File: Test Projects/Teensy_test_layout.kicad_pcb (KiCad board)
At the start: 2 copper layers, 203.2 x 101.6 mm, 106 parts, among them P1 CONN_01X02, P10 CONN_01X08, P11 CONN_01X08, P12 COLUMNS, P13 CONN_01X08, P14 CONN_01X08, P15 CONN_01X08, P16 CONN_01X08, P17 CONN_01X08, P18 CONN_01X08, P19 CONN_01X08, P2 CONN_01X07, P20 CONN_01X08, P3 CONN_01X08, P4 CONN_01X08, P5 CONN_01X08, P6 CONN_01X08, P7 ROWS, P8 CONN_01X08, P9 CONN_01X08, U1 LDO-adj-4term, U10 SF-4052, U11 SF-4052, U12 SF-4052, U13 SF-4052, U14 SF-4052, U15 SF-4052, U16 SF-4052, U17 SF-4052, U18 SF-74HC595, U19 SF-74HC595, U2 Teensy_3.2, U20 SF-74HC595, U21 SF-74HC595, U22 SF-74HC595, U23 SF-74HC595, U24 SF-74HC595, U25 SF-74HC595, U26 SF-74HC595, U27 SF-74HC595, U3 LDO-adj-4term, U4 SGTL5000, U5 SF-MicroSD-12term, U6 LDO-adj-4term, U7 2N168, U8 SF-4052, U9 SF-4052

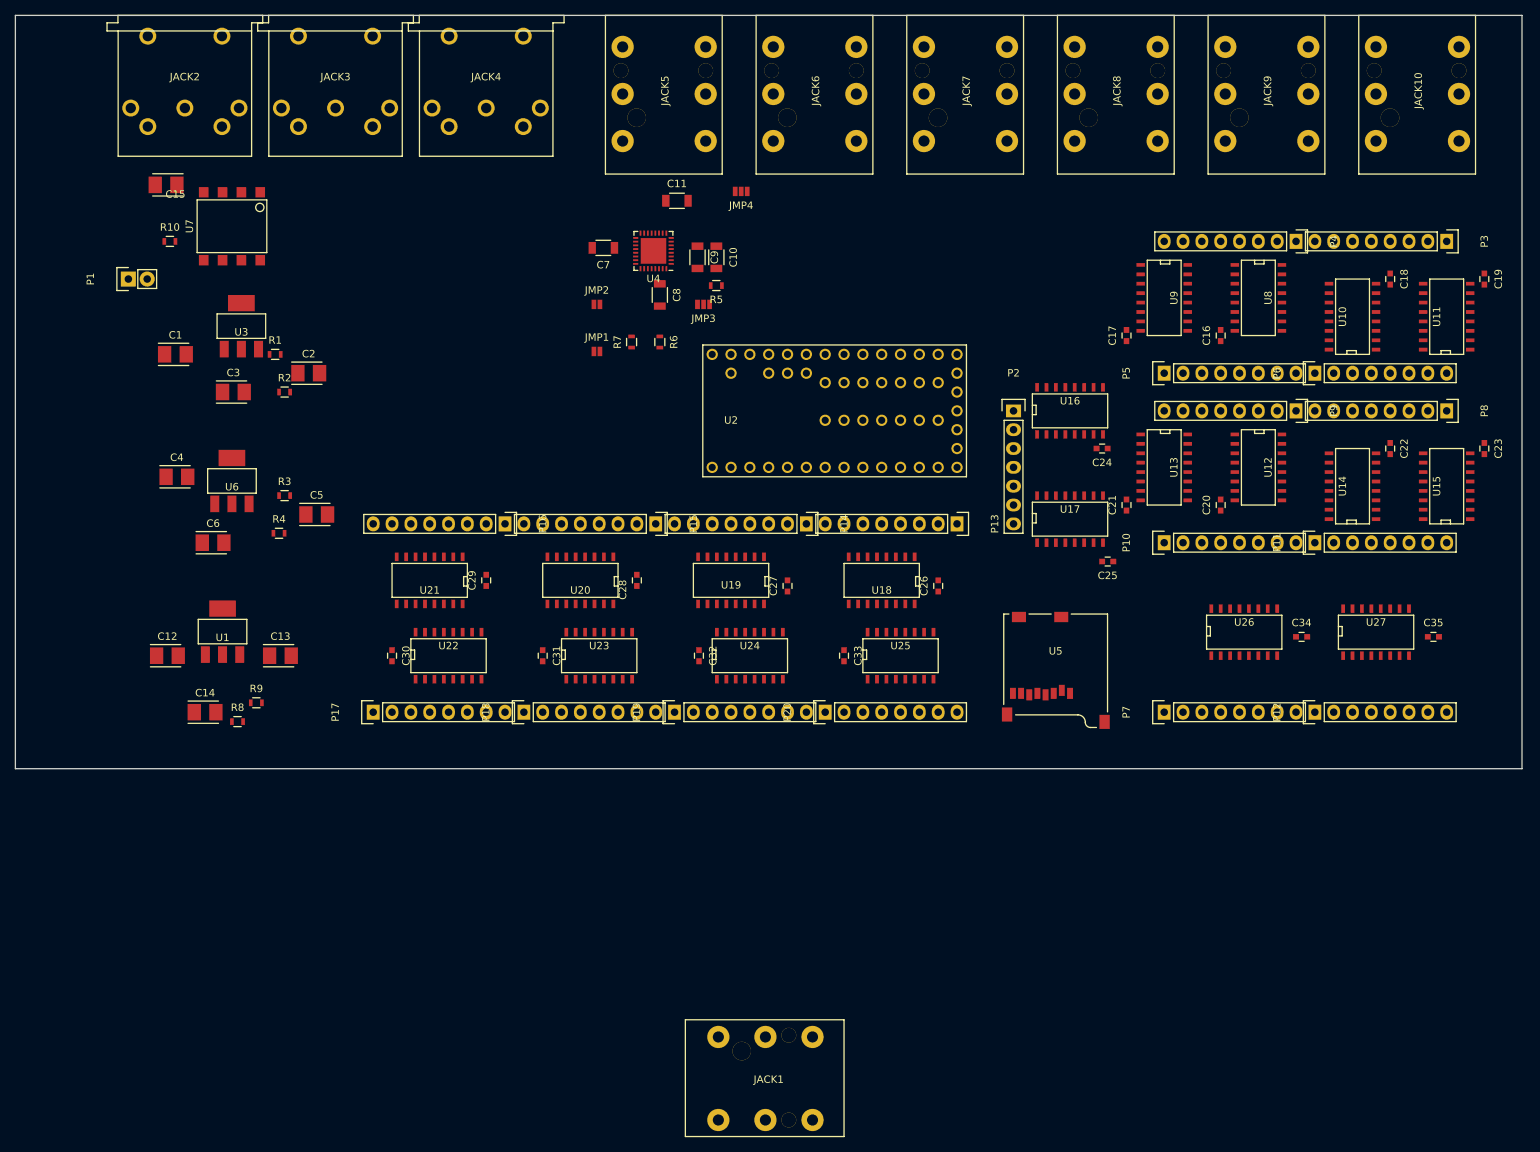
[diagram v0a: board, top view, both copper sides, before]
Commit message: Tested a few layout sections
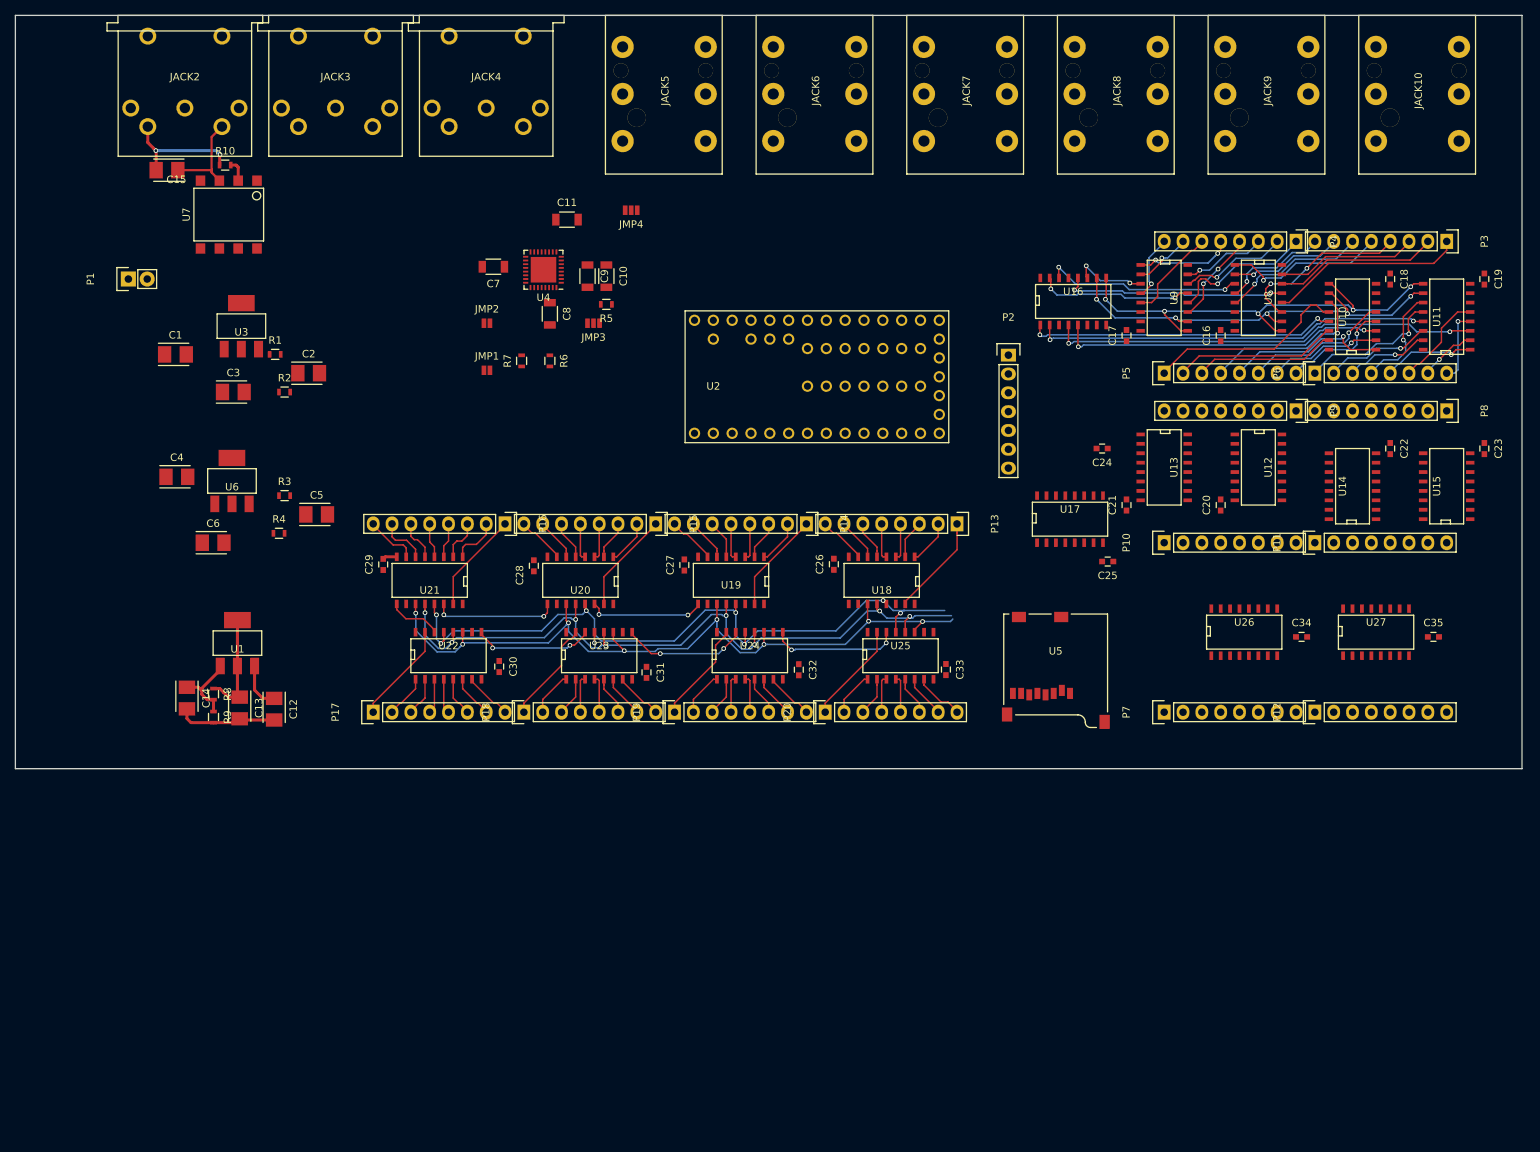
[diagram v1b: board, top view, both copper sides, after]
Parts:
- removed JACK1: TRS_6term, SparkFun-Footprints:SF-Neutrik-Jack-6-term
- moved C12 16.1 mm to (85.7, 131.7), turned to 270 degrees
- moved R5 15.0 mm to (130.5, 77.1)
- moved C10 15.0 mm to (130.5, 73.3)
- moved C9 15.0 mm to (128.0, 73.3)
- moved JMP4 15.0 mm to (133.9, 64.4)
- moved JMP1 15.0 mm to (114.4, 86.0)
- moved JMP2 15.0 mm to (114.4, 79.6)
- moved R6 15.0 mm to (122.9, 84.7)
- moved R7 15.0 mm to (119.1, 84.7)
- moved C11 15.0 mm to (125.2, 65.6)
- moved C8 15.0 mm to (122.9, 78.3)
- moved C7 15.0 mm to (115.3, 72.0)
- moved JMP3 15.0 mm to (128.8, 79.6)
- moved U4 15.0 mm to (122.0, 72.4)
- moved U16 14.8 mm to (193.5, 76.7)
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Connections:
- net Net-(C1-Pad1) renamed /page1/Bulk_IN
- U10 pad 13: (no net) -> KOUT5
- U10 pad 3: (no net) -> KOUT6
- U11 pad 13: (no net) -> KOUT7
- U11 pad 3: (no net) -> KOUT8
- U16 pad 1: (no net) -> KOUT5
- U16 pad 11: (no net) -> KOUT4
- U16 pad 12: (no net) -> KOUT1
- U16 pad 14: (no net) -> KOUT2
- U16 pad 15: (no net) -> KOUT3
- U16 pad 2: (no net) -> KOUT7
- U16 pad 4: (no net) -> KOUT8
- U16 pad 5: (no net) -> KOUT6
- U18 pad 14: BSER -> LEDSER
- U2 pad 28: (no net) -> BCLK
- U2 pad 29: BCLK -> (no net)
- U2 pad 31: (no net) -> LEDSER
- U8 pad 13: (no net) -> KOUT1
- U8 pad 3: (no net) -> KOUT2
- U9 pad 13: (no net) -> KOUT3
- U9 pad 3: (no net) -> KOUT4
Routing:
- net LEDSCLK: track 0.00 -> 102.9 mm, vias 0 -> 8
- net LEDLATCH: track 0.00 -> 101.0 mm, vias 0 -> 8
- net LEDOE: track 0.00 -> 99.2 mm, vias 0 -> 8
- net B: track 0.00 -> 62.6 mm, vias 0 -> 5
- net A: track 0.00 -> 58.4 mm, vias 0 -> 5
- net KOUT8: track 0.00 -> 58.2 mm, vias 0 -> 2
- net KOUT7: track 0.00 -> 53.8 mm, vias 0 -> 2
- net KOUT6: track 0.00 -> 44.3 mm, vias 0 -> 2
- net KOUT5: track 0.00 -> 41.6 mm, vias 0 -> 2
- net KOUT1: track 0.00 -> 30.2 mm, vias 0 -> 2
- net K17: track 0.00 -> 27.1 mm
- net KOUT2: track 0.00 -> 26.8 mm, vias 0 -> 2
- net K1: track 0.00 -> 26.4 mm
- net K4: track 0.00 -> 23.7 mm, vias 0 -> 2
- net K20: track 0.00 -> 22.9 mm, vias 0 -> 1
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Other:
- net class Default: clearance 0.2 -> 0.1778; trace_width 0.25 -> 0.1778; via_dia 0.6 -> 0.635; via_drill 0.4 -> 0.381
- net class JackLine added: clearance 0.3048, trace_width 0.3048, via_dia 0.635, via_drill 0.381
- net class Power added: clearance 0.254, trace_width 0.4064, via_dia 0.635, via_drill 0.381
- net class Signal added: clearance 0.254, trace_width 0.2032, via_dia 0.635, via_drill 0.381
- rule trace_clearance: 0.2 -> 0.1778
- rule trace_min: 0.2 -> 0.1778
- rule via_min_drill: 0.3 -> 0.381
- rule via_min_size: 0.4 -> 0.508

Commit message: Continued proto 1 layout
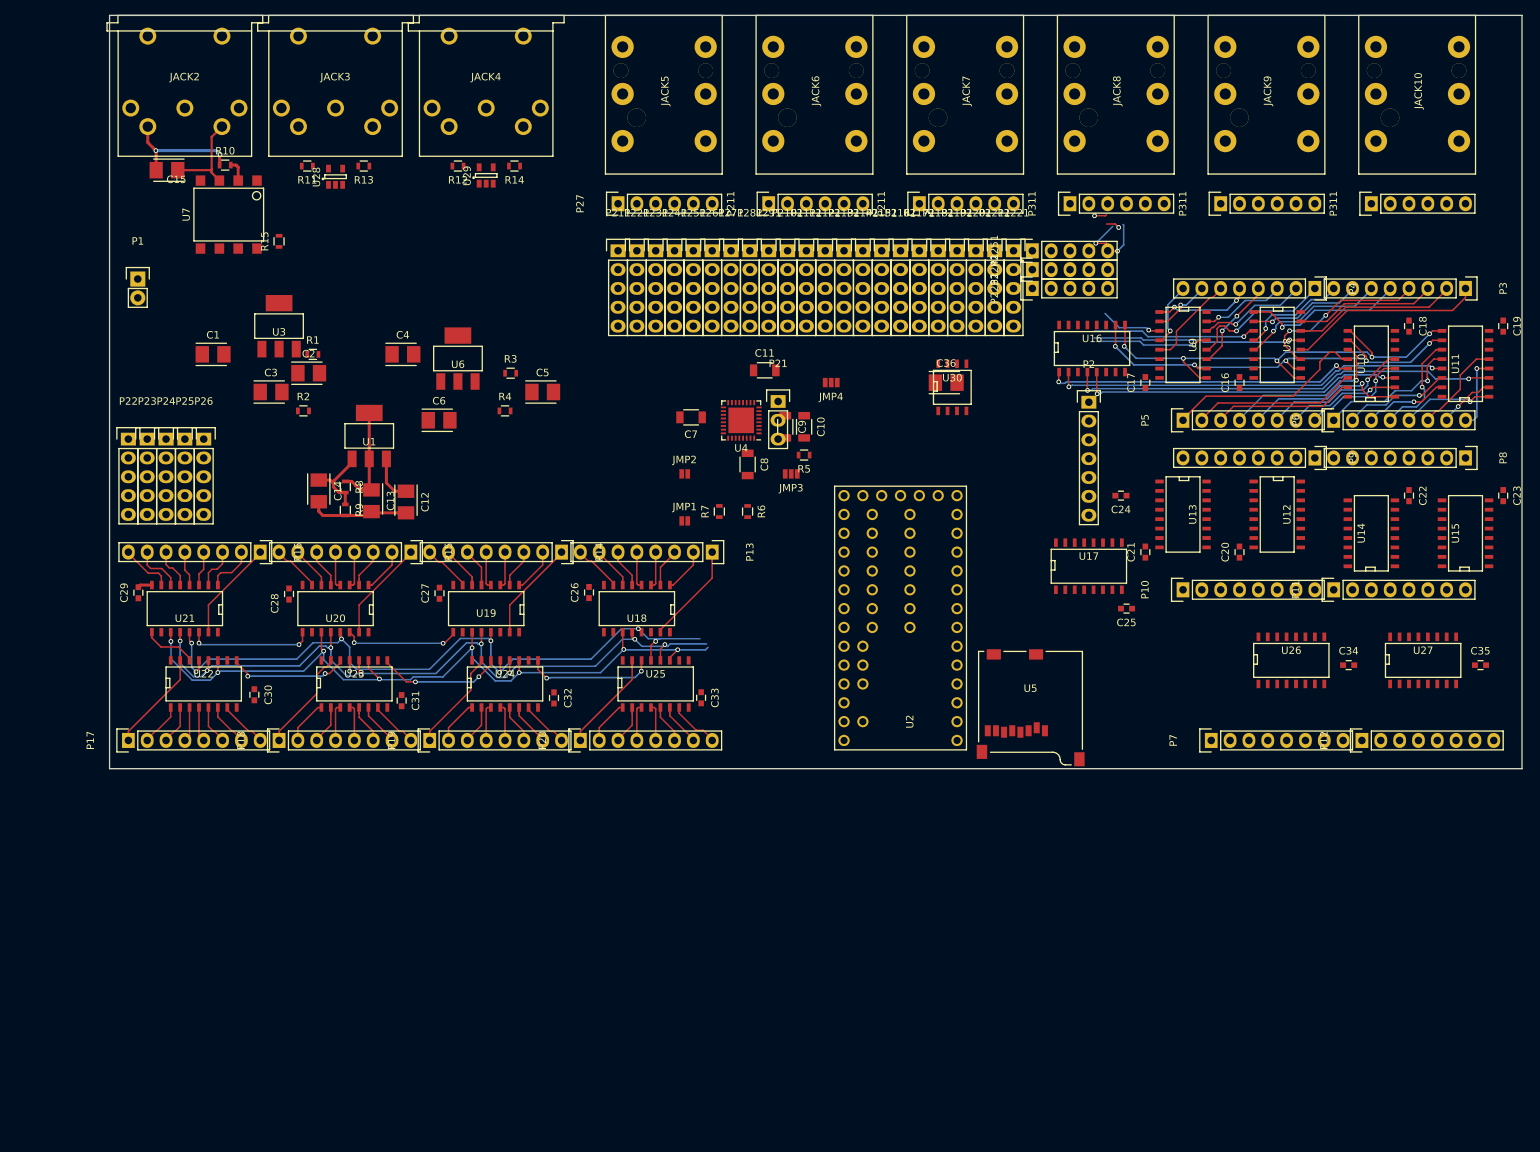
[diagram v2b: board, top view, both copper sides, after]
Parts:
- added C36: C, Capacitors_Tantalum_SMD:TantalC_SizeB_EIA-3528_Reflow, F.Cu at (176.3, 87.6)
- added P21: CONN_01X03, Pin_Headers:Pin_Header_Straight_1x03, F.Cu at (153.7, 90.2)
- added P2101: CONN_01X05, Pin_Headers:Pin_Header_Straight_1x05, F.Cu at (154.9, 69.8)
- added P211: CONN_01X05, Pin_Headers:Pin_Header_Straight_1x05, F.Cu at (132.1, 69.8)
- added P211: CONN_01X06, Pin_Headers:Pin_Header_Straight_1x06, F.Cu at (152.4, 63.5)
- added P211: CONN_01X06, Pin_Headers:Pin_Header_Straight_1x06, F.Cu at (172.7, 63.5)
- added P2111: CONN_01X05, Pin_Headers:Pin_Header_Straight_1x05, F.Cu at (157.5, 69.8)
- added P2121: CONN_01X05, Pin_Headers:Pin_Header_Straight_1x05, F.Cu at (160.0, 69.8)
- added P2131: CONN_01X05, Pin_Headers:Pin_Header_Straight_1x05, F.Cu at (162.6, 69.8)
- added P2141: CONN_01X05, Pin_Headers:Pin_Header_Straight_1x05, F.Cu at (165.1, 69.8)
- added P2151: CONN_01X05, Pin_Headers:Pin_Header_Straight_1x05, F.Cu at (167.6, 69.8)
- added P2161: CONN_01X05, Pin_Headers:Pin_Header_Straight_1x05, F.Cu at (170.2, 69.8)
- added P2171: CONN_01X05, Pin_Headers:Pin_Header_Straight_1x05, F.Cu at (172.7, 69.8)
- added P2181: CONN_01X05, Pin_Headers:Pin_Header_Straight_1x05, F.Cu at (175.3, 69.8)
- added P2191: CONN_01X05, Pin_Headers:Pin_Header_Straight_1x05, F.Cu at (177.8, 69.8)
- added P22: CONN_01X05, Pin_Headers:Pin_Header_Straight_1x05, F.Cu at (66.0, 95.2)
- added P2201: CONN_01X05, Pin_Headers:Pin_Header_Straight_1x05, F.Cu at (180.3, 69.8)
- added P221: CONN_01X05, Pin_Headers:Pin_Header_Straight_1x05, F.Cu at (134.6, 69.8)
- added P2211: CONN_01X05, Pin_Headers:Pin_Header_Straight_1x05, F.Cu at (182.9, 69.8)
- added P2221: CONN_01X05, Pin_Headers:Pin_Header_Straight_1x05, F.Cu at (185.4, 69.8)
- added P2231: CONN_01X05, Pin_Headers:Pin_Header_Straight_1x05, F.Cu at (188.0, 74.9)
- added P2241: CONN_01X05, Pin_Headers:Pin_Header_Straight_1x05, F.Cu at (188.0, 72.4)
- added P2251: CONN_01X05, Pin_Headers:Pin_Header_Straight_1x05, F.Cu at (188.0, 69.8)
- added P23: CONN_01X05, Pin_Headers:Pin_Header_Straight_1x05, F.Cu at (68.6, 95.2)
- added P231: CONN_01X05, Pin_Headers:Pin_Header_Straight_1x05, F.Cu at (137.2, 69.8)
- added P24: CONN_01X05, Pin_Headers:Pin_Header_Straight_1x05, F.Cu at (71.1, 95.2)
- added P241: CONN_01X05, Pin_Headers:Pin_Header_Straight_1x05, F.Cu at (139.7, 69.8)
- added P25: CONN_01X05, Pin_Headers:Pin_Header_Straight_1x05, F.Cu at (73.7, 95.2)
- added P251: CONN_01X05, Pin_Headers:Pin_Header_Straight_1x05, F.Cu at (142.2, 69.8)
- added P26: CONN_01X05, Pin_Headers:Pin_Header_Straight_1x05, F.Cu at (76.2, 95.2)
- added P261: CONN_01X05, Pin_Headers:Pin_Header_Straight_1x05, F.Cu at (144.8, 69.8)
- added P27: CONN_01X06, Pin_Headers:Pin_Header_Straight_1x06, F.Cu at (132.1, 63.5)
- added P271: CONN_01X05, Pin_Headers:Pin_Header_Straight_1x05, F.Cu at (147.3, 69.8)
- added P281: CONN_01X05, Pin_Headers:Pin_Header_Straight_1x05, F.Cu at (149.9, 69.8)
- added P291: CONN_01X05, Pin_Headers:Pin_Header_Straight_1x05, F.Cu at (152.4, 69.8)
- added P311: CONN_01X06, Pin_Headers:Pin_Header_Straight_1x06, F.Cu at (193.0, 63.5)
- added P311: CONN_01X06, Pin_Headers:Pin_Header_Straight_1x06, F.Cu at (213.4, 63.5)
- added P311: CONN_01X06, Pin_Headers:Pin_Header_Straight_1x06, F.Cu at (233.7, 63.5)
- added R11: R, Resistors_SMD:R_0603, F.Cu at (90.2, 58.4)
- added R12: R, Resistors_SMD:R_0603, F.Cu at (110.5, 58.4)
- added R13: R, Resistors_SMD:R_0603, F.Cu at (97.8, 58.4)
- added R14: R, Resistors_SMD:R_0603, F.Cu at (118.1, 58.4)
- added R15: R, Resistors_SMD:R_0603, F.Cu at (86.4, 68.6)
- added U28: SF-74x125, SparkFun-Footprints:SF-SOT-23-5, F.Cu at (94.0, 59.9)
- added U29: SF-74x125, SparkFun-Footprints:SF-SOT-23-5, F.Cu at (114.3, 59.7)
- added U30: SF-LM358, SparkFun-Footprints:SF-SOIC-8, F.Cu at (177.2, 88.3)
- P12: value COLUMNS -> COLS1
- P7: value ROWS -> COLS0
- moved JMP4 35.6 mm to (160.8, 87.6)
- moved C4 34.7 mm to (103.1, 83.8)
- moved C6 34.7 mm to (108.0, 92.7)
- moved R3 34.7 mm to (117.6, 86.4)
- moved R4 34.7 mm to (116.8, 91.4)
- moved C5 34.7 mm to (121.9, 88.9)
- moved U6 34.7 mm to (110.5, 84.4)
- moved U2 34.4 mm to (170.2, 119.4), turned to 180 degrees
- moved C10 33.5 mm to (157.2, 93.6)
- moved C9 33.5 mm to (154.6, 93.6)
- moved R5 33.5 mm to (157.2, 97.4)
- moved C11 33.5 mm to (151.9, 86.0)
- moved C8 33.5 mm to (149.6, 98.7)
- moved JMP1 33.5 mm to (141.1, 106.3)
- moved JMP2 33.5 mm to (141.1, 99.9)
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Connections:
- C26 pad 1: Net-(C26-Pad1) -> +5V
- C26 pad 2: Net-(C26-Pad2) -> GND
- C27 pad 1: Net-(C27-Pad1) -> +5V
- C27 pad 2: Net-(C27-Pad2) -> GND
- C28 pad 1: Net-(C28-Pad1) -> +5V
- C28 pad 2: Net-(C28-Pad2) -> GND
- C29 pad 1: Net-(C29-Pad1) -> +5V
- C29 pad 2: Net-(C29-Pad2) -> GND
- C30 pad 1: Net-(C30-Pad1) -> +5V
- C30 pad 2: Net-(C30-Pad2) -> GND
- C31 pad 1: Net-(C31-Pad1) -> +5V
- C31 pad 2: Net-(C31-Pad2) -> GND
- C32 pad 1: Net-(C32-Pad1) -> +5V
- C32 pad 2: Net-(C32-Pad2) -> GND
- C33 pad 1: Net-(C33-Pad1) -> +5V
- C33 pad 2: Net-(C33-Pad2) -> GND
- JACK10 pad G: (no net) -> Net-(JACK10-PadG)
- JACK10 pad R: (no net) -> Net-(JACK10-PadR)
- JACK10 pad RN: (no net) -> Net-(JACK10-PadRN)
- JACK10 pad S: (no net) -> Net-(JACK10-PadS)
- JACK10 pad T: (no net) -> Net-(JACK10-PadT)
- JACK10 pad TN: (no net) -> Net-(JACK10-PadTN)
- JACK3 pad 4: (no net) -> Net-(JACK3-Pad4)
- JACK3 pad 5: (no net) -> Net-(JACK3-Pad5)
- JACK4 pad 4: (no net) -> Net-(JACK4-Pad4)
- JACK4 pad 5: (no net) -> Net-(JACK4-Pad5)
- JACK5 pad G: (no net) -> Net-(JACK5-PadG)
- JACK5 pad R: (no net) -> Net-(JACK5-PadR)
- JACK5 pad RN: (no net) -> Net-(JACK5-PadRN)
- JACK5 pad S: (no net) -> Net-(JACK5-PadS)
- JACK5 pad T: (no net) -> Net-(JACK5-PadT)
- JACK5 pad TN: (no net) -> Net-(JACK5-PadTN)
- JACK6 pad G: (no net) -> Net-(JACK6-PadG)
- JACK6 pad R: (no net) -> Net-(JACK6-PadR)
- JACK6 pad RN: (no net) -> Net-(JACK6-PadRN)
- JACK6 pad S: (no net) -> Net-(JACK6-PadS)
- JACK6 pad T: (no net) -> Net-(JACK6-PadT)
- JACK6 pad TN: (no net) -> Net-(JACK6-PadTN)
- JACK7 pad G: (no net) -> Net-(JACK7-PadG)
- JACK7 pad R: (no net) -> Net-(JACK7-PadR)
- JACK7 pad RN: (no net) -> Net-(JACK7-PadRN)
- JACK7 pad S: (no net) -> Net-(JACK7-PadS)
- JACK7 pad T: (no net) -> Net-(JACK7-PadT)
- JACK7 pad TN: (no net) -> Net-(JACK7-PadTN)
- JACK8 pad G: (no net) -> Net-(JACK8-PadG)
- JACK8 pad R: (no net) -> Net-(JACK8-PadR)
- JACK8 pad RN: (no net) -> Net-(JACK8-PadRN)
- JACK8 pad S: (no net) -> Net-(JACK8-PadS)
- JACK8 pad T: (no net) -> Net-(JACK8-PadT)
- JACK8 pad TN: (no net) -> Net-(JACK8-PadTN)
- JACK9 pad G: (no net) -> Net-(JACK9-PadG)
- JACK9 pad R: (no net) -> Net-(JACK9-PadR)
- JACK9 pad RN: (no net) -> Net-(JACK9-PadRN)
- JACK9 pad S: (no net) -> Net-(JACK9-PadS)
- JACK9 pad T: (no net) -> Net-(JACK9-PadT)
- JACK9 pad TN: (no net) -> Net-(JACK9-PadTN)
- P2 pad 5: (no net) -> KEN
- U18 pad 16: Net-(C26-Pad1) -> +5V
- U18 pad 8: Net-(C26-Pad2) -> GND
- U19 pad 16: Net-(C27-Pad1) -> +5V
- U19 pad 8: Net-(C27-Pad2) -> GND
- U2 pad 21: (no net) -> KEN
- U20 pad 16: Net-(C28-Pad1) -> +5V
- U20 pad 8: Net-(C28-Pad2) -> GND
- U21 pad 16: Net-(C29-Pad1) -> +5V
- U21 pad 8: Net-(C29-Pad2) -> GND
- U22 pad 16: Net-(C30-Pad1) -> +5V
- U22 pad 8: Net-(C30-Pad2) -> GND
- U23 pad 16: Net-(C31-Pad1) -> +5V
- U23 pad 8: Net-(C31-Pad2) -> GND
- U24 pad 16: Net-(C32-Pad1) -> +5V
- U24 pad 8: Net-(C32-Pad2) -> GND
- U25 pad 16: Net-(C33-Pad1) -> +5V
- U25 pad 8: Net-(C33-Pad2) -> GND
- U7 pad 5: (no net) -> GND
- U7 pad 6: (no net) -> PORT-TX
- U7 pad 8: (no net) -> +5V
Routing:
- net Net-(C29-Pad2): track 1.94 -> 0.00 mm
- net GND: track 13.6 -> 15.5 mm
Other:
- board size 203.2 x 101.6 mm -> 190.5 x 101.6 mm
